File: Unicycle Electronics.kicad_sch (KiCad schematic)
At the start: 18 parts, among them Q1 2N7002, SW1 INSERT PART NUMBER, SW2 INSERT PART NUMBER, U1 LDH-65-700, U2 ESP32-C6-MINI-1/U, U3 AMS1117-3.3

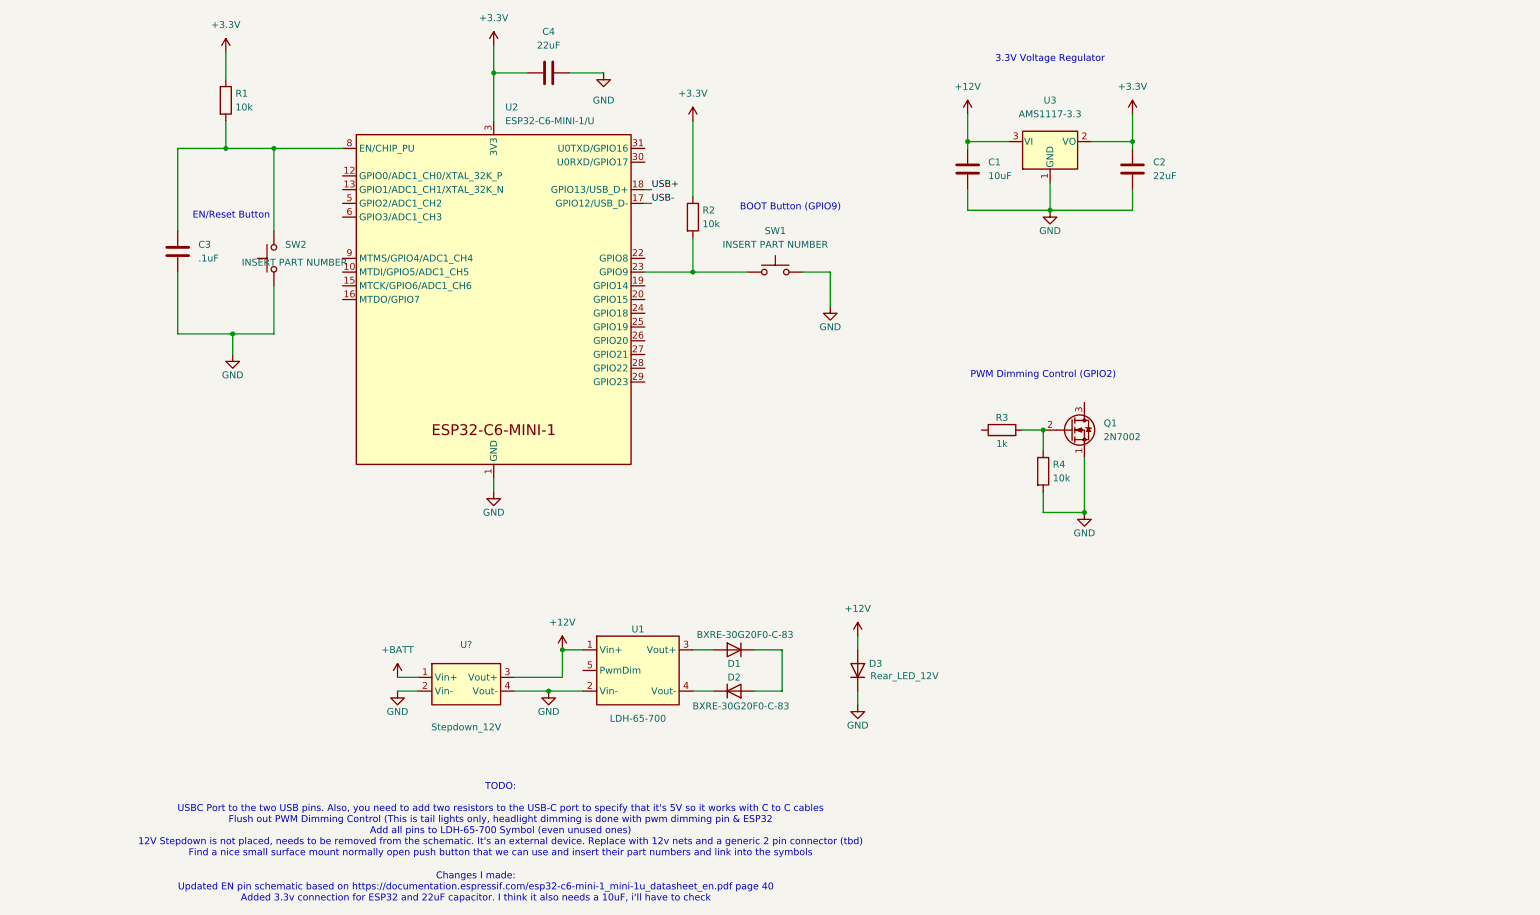
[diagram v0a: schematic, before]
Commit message: Schematic Update
Worked on some TODO List
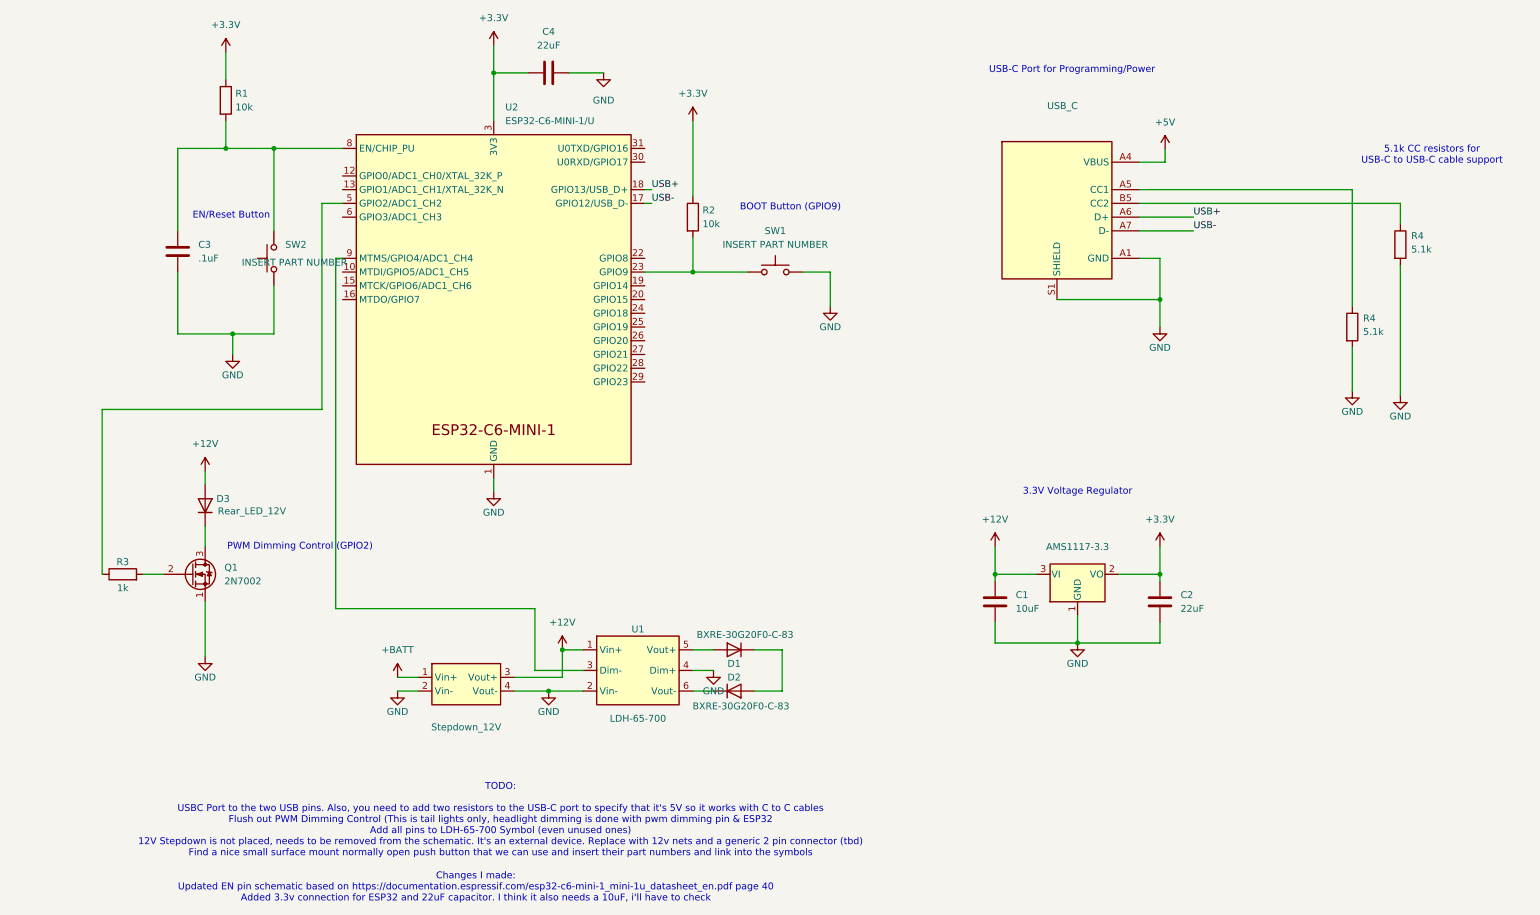
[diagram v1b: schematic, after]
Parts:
- removed R4: 10k, symbol Device:R
- added J1: USB_C, symbol Connector:USB_C_Receptacle_USB2.0
- added R4 (x2): 5.1k, symbol Device:R
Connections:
- net GND: now also U1.4 (Dim+), J1.A1 (GND), J1.A12 (GND), J1.B1 (GND), J1.B12 (GND), J1.S1 (SHIELD), R4.2, R4.2; no longer D3.1 (A)
- net USB+: now also J1.A6 (D+), J1.B6 (D+)
- net USB-: now also J1.A7 (D-), J1.B7 (D-)
- net at Q1.3 (D): now also D3.1 (A)
- net at D2.2 (K): now also U1.5 (Vout+); no longer U1.3 (Vout+)
- net at R3.1: now also U2.5 (GPIO2/ADC1_CH2)
- net at D1.1 (A): now also U1.6 (Vout-); no longer U1.4 (Vout-)
- net at U2.9 (MTMS/GPIO4/ADC1_CH4): now also U1.3 (Dim-)
- new net: J1.A5 (CC1), R4.1
- new net: J1.B5 (CC2), R4.1
- new net +5V: J1.A4 (VBUS), J1.A9 (VBUS), J1.B4 (VBUS), J1.B9 (VBUS)
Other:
- note added: "5.1k CC resistors for USB-C to USB-C cable support"
- note added: "USB-C Port for Programming/Power"
- moved on the sheet: C1, C2, D3, Q1, R3
